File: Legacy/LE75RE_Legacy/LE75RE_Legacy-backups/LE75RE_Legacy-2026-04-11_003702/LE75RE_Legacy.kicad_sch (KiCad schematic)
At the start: 179 parts, among them P1 USB_C_Plug_USB2.0, SW1 SW_Push, U1 MCP1703Ax-330xxDB, U2 STM32F072CBTx

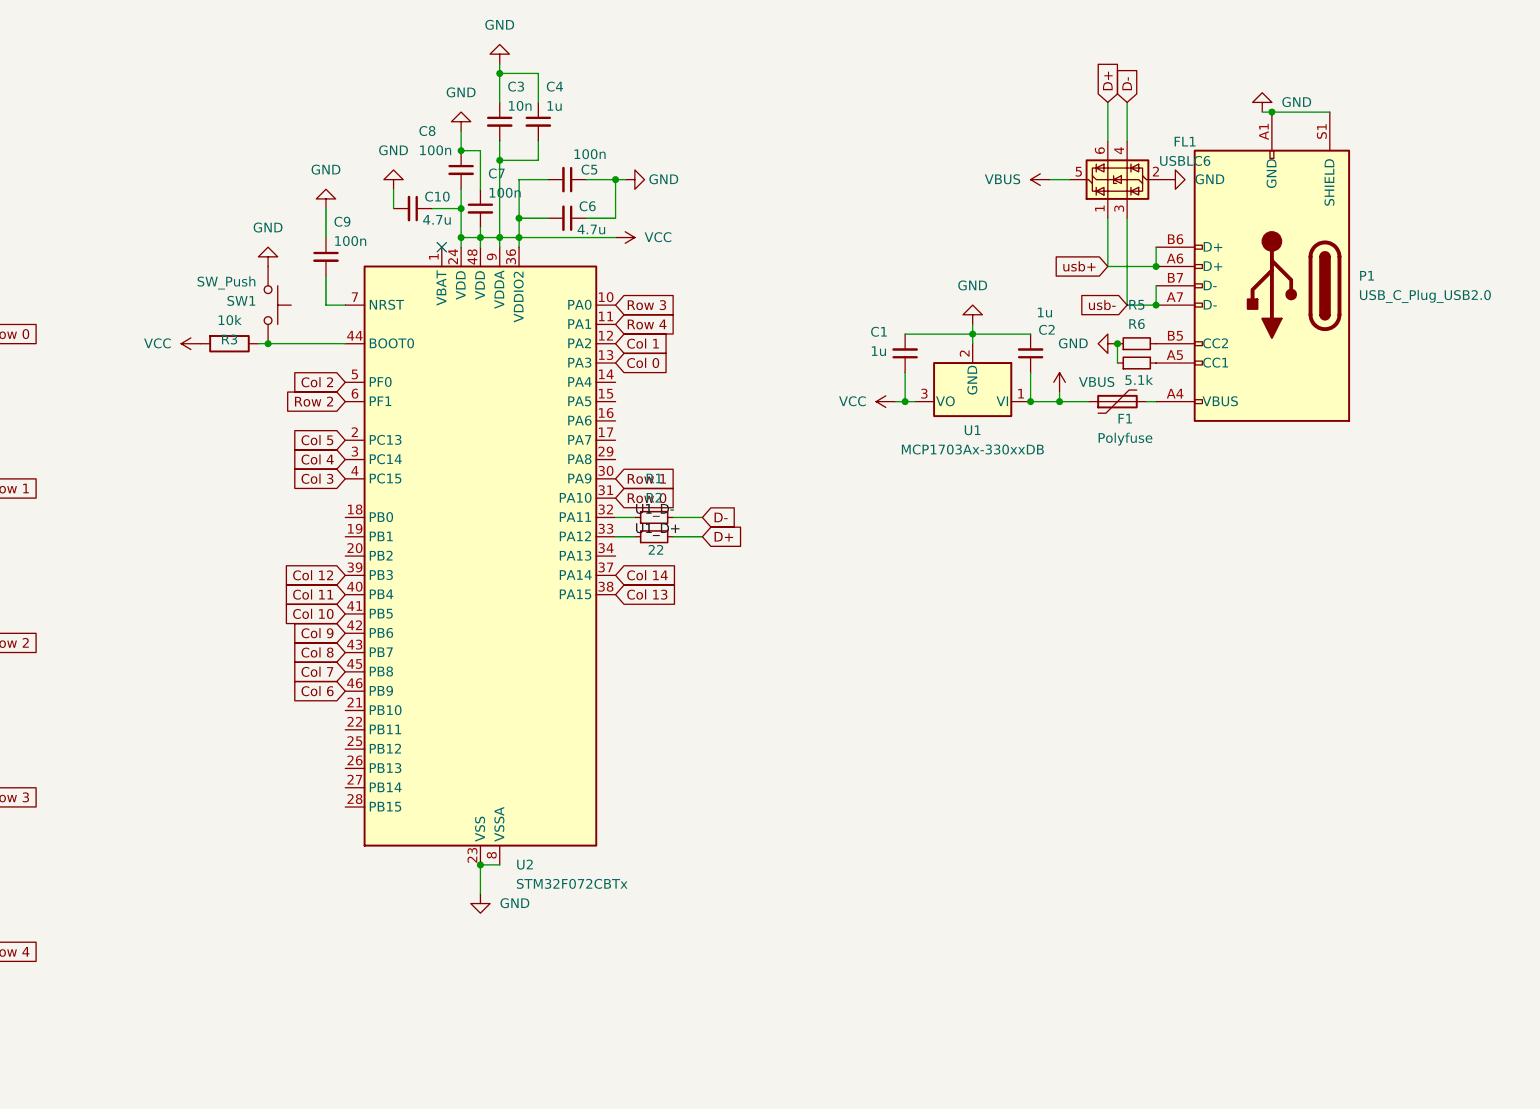
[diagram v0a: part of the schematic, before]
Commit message: Many changes
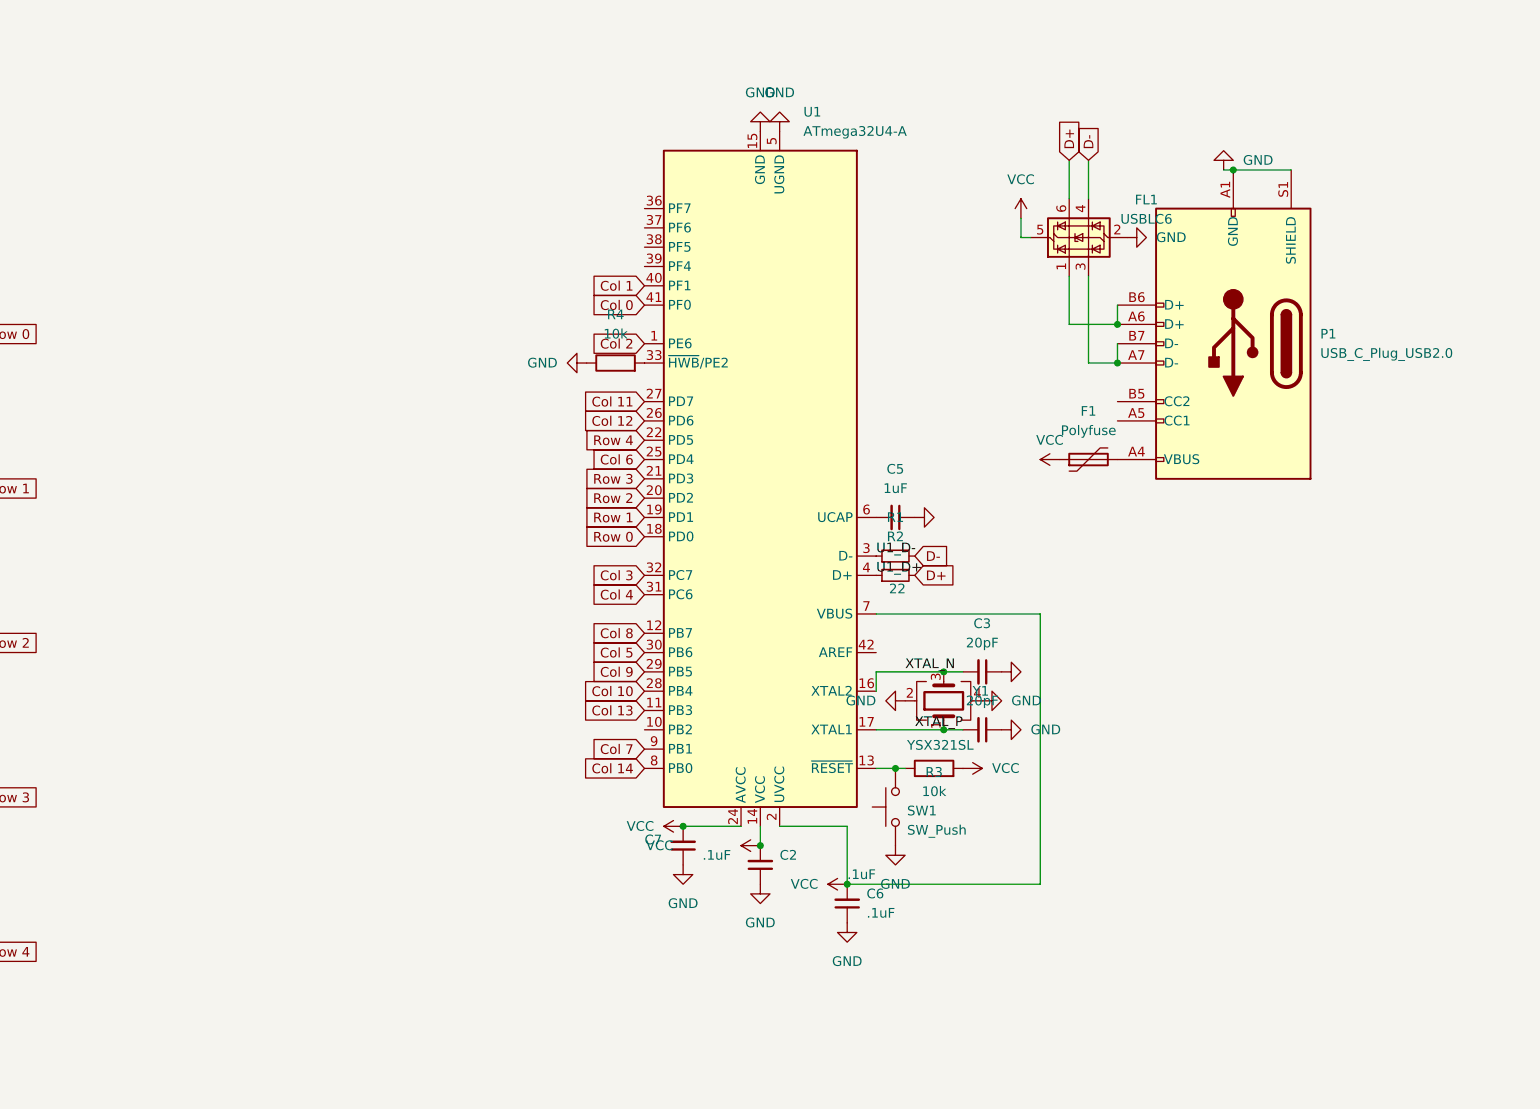
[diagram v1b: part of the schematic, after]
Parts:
- removed C1: 1u, Capacitor_SMD:C_0603_1608Metric, symbol Device:C_Small
- removed C10: 4.7u, Capacitor_SMD:C_0603_1608Metric, symbol Device:C_Small
- removed C8, C9: 100n, Capacitor_SMD:C_0603_1608Metric, symbol Device:C_Small
- removed R5, R6: 5.1k, Resistor_SMD:R_0603_1608Metric, symbol Device:R_Small
- removed U1: MCP1703Ax-330xxDB, Package_TO_SOT_SMD:SOT-223-3_TabPin2, symbol Regulator_Linear:MCP1703Ax-330xxDB
- removed U2: STM32F072CBTx, Package_QFP:LQFP-48_7x7mm_P0.5mm, symbol MCU_ST_STM32F0:STM32F072CBTx
- added R4: 10k, Resistor_SMD:R_0603_1608Metric, symbol Device:R
- added U1: ATmega32U4-A, Package_DFN_QFN:QFN-44-1EP_7x7mm_P0.5mm_EP5.2x5.2mm, symbol MCU_Microchip_ATmega:ATmega32U4-M
- added Y1: YSX321SL, Crystal:Crystal_SMD_3225-4Pin_3.2x2.5mm, symbol Device:Crystal_GND24
- C2: value 1u -> .1uF
- C3: value 10n -> 20pF
- C4: value 1u -> 20pF
- C5: value 100n -> 1uF
- C6: value 4.7u -> .1uF
- C7: value 100n -> .1uF
- S1, S10, S11, S12, S13, S14, S15, S16, S17, S18, S19, S2, S20, S21, S22, S23, S24, S25, S26, S27, S28, S29, S3, S30, S31, S32, S33, S34, S35, S36, S37, S38, S39, S4, S40, S41, S42, S43, S44, S45, S46, S47, S48, S49, S5, S50, S51, S52, S53, S54, S55, S56, S57, S58, S59, S6, S60, S61, S62, S63, S64, S65, S66, S67, S68, S69, S7, S70, S71, S72, S73, S74, S75, S8, S9: footprint Gateron_KS33_Hotswap:Gateron-KS33-Hotswap-1U -> PCM_Switch_Keyboard_Hotswap_Kailh:SW_Hotswap_Kailh_MX_Plated
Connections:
- net Col 0: now also U1.41 (PF0)
- net Col 1: now also U1.40 (PF1)
- net Col 10: now also U1.28 (PB4)
- net Col 11: now also U1.27 (PD7)
- net Col 12: now also U1.26 (PD6)
- net Col 13: now also U1.11 (PB3)
- net Col 14: now also U1.8 (PB0)
- net Col 2: now also U1.1 (PE6)
- net Col 3: now also U1.32 (PC7)
- net Col 4: now also U1.31 (PC6)
- net Col 5: now also U1.30 (PB6)
- net Col 6: now also U1.25 (PD4)
- net Col 7: now also U1.9 (PB1)
- net Col 8: now also U1.12 (PB7)
- net Col 9: now also U1.29 (PB5)
- net GND: now also C2.1, R4.1, U1.15 (GND), U1.23 (GND), U1.35 (GND), U1.43 (GND), U1.45 (GND), U1.5 (UGND), Y1.2, Y1.4; no longer C2.2
- net Row 0: now also U1.18 (PD0)
- net Row 1: now also U1.19 (PD1)
- net Row 2: now also U1.20 (PD2)
- net Row 3: now also U1.21 (PD3)
- net Row 4: now also U1.22 (PD5)
- net U1_D+: now also U1.4 (D+)
- net U1_D-: now also U1.3 (D-)
- net VCC: now also C2.2, F1.1, FL1.5 (VBUS), U1.14 (VCC), U1.2 (UVCC), U1.24 (AVCC), U1.34 (VCC), U1.44 (AVCC), U1.7 (VBUS); no longer C3.2, C4.2, C5.2
- net at R3.1, SW1.2: now also U1.13 (~{RESET})
- removed net VBUS: C2.1, F1.1, FL1.5 (VBUS)
- net usb+: no longer names the net of FL1.1 (I/O1), P1.A6 (D+), P1.B6 (D+)
- net usb-: no longer names the net of FL1.3 (I/O2), P1.A7 (D-), P1.B7 (D-)
- new net: C5.2, U1.6 (UCAP)
- new net: R4.2, U1.33 (~{HWB}/PE2)
- new net XTAL_N: C3.2, U1.16 (XTAL2), Y1.3
- new net XTAL_P: C4.2, U1.17 (XTAL1), Y1.1
- no-connect marks 1 -> 0
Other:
- moved on the sheet: F1, FL1, P1, R1, R2, R3, SW1
